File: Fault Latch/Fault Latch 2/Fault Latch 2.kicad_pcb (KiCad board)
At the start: 2 copper layers, 9 parts, among them K103 Fujitsu_FTR-LYAA005x, K104 Fujitsu_FTR-LYAA005x, K105 Fujitsu_FTR-LYAA005x, SW1 SW_Omron_B3FS, SW2 SW_Omron_B3FS, SW3 SW_Omron_B3FS, U105 SFH617A-1, U108 SFH617A-1, U111 SFH617A-1

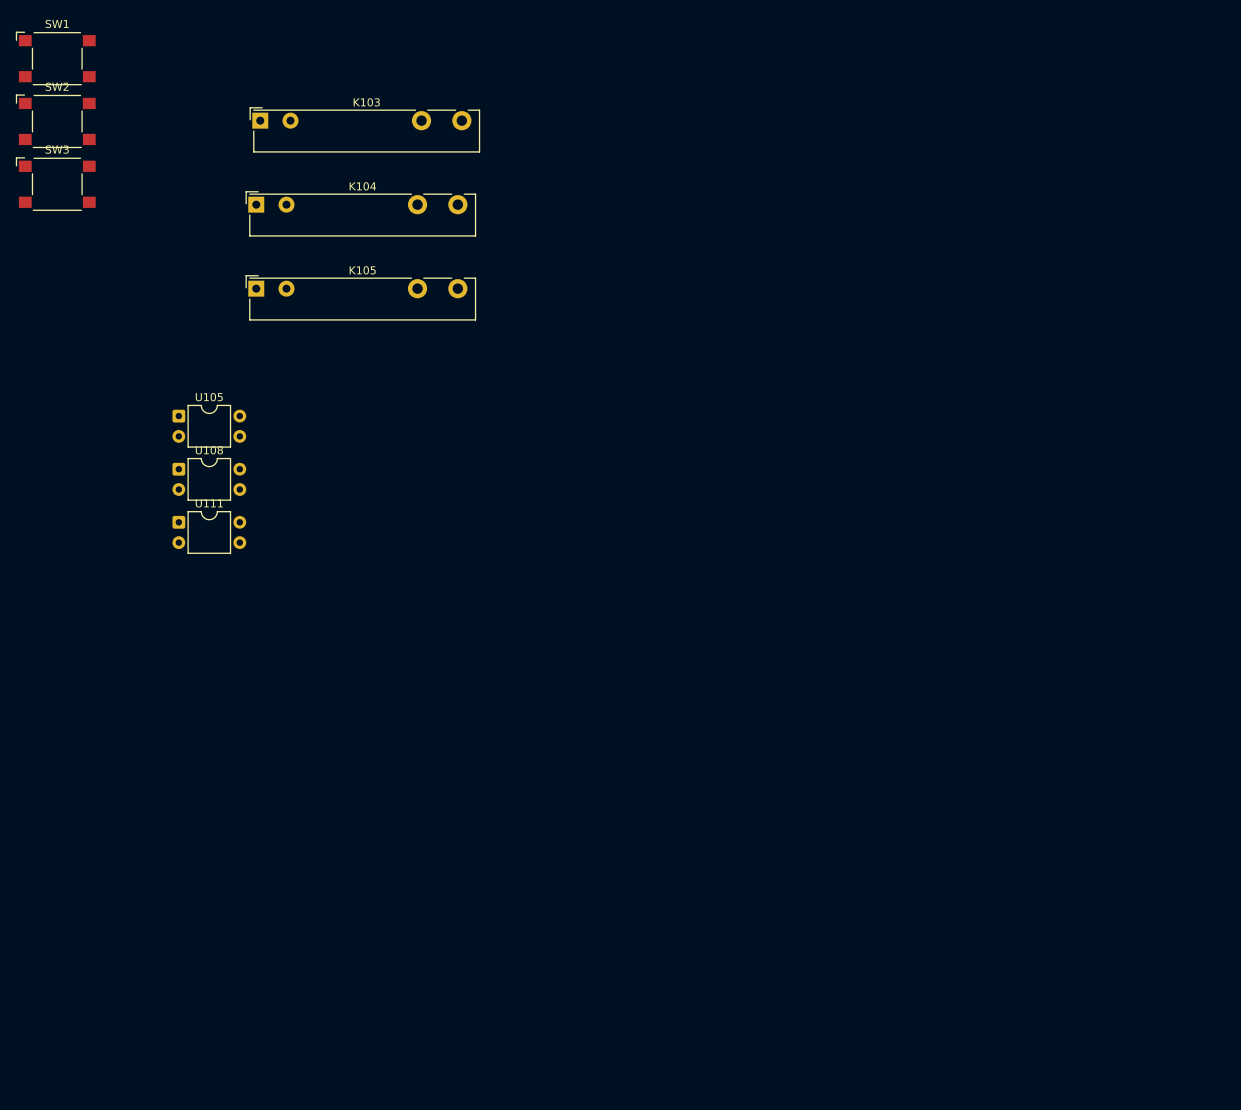
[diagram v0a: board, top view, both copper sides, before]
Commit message: Fault Latch Overhaul
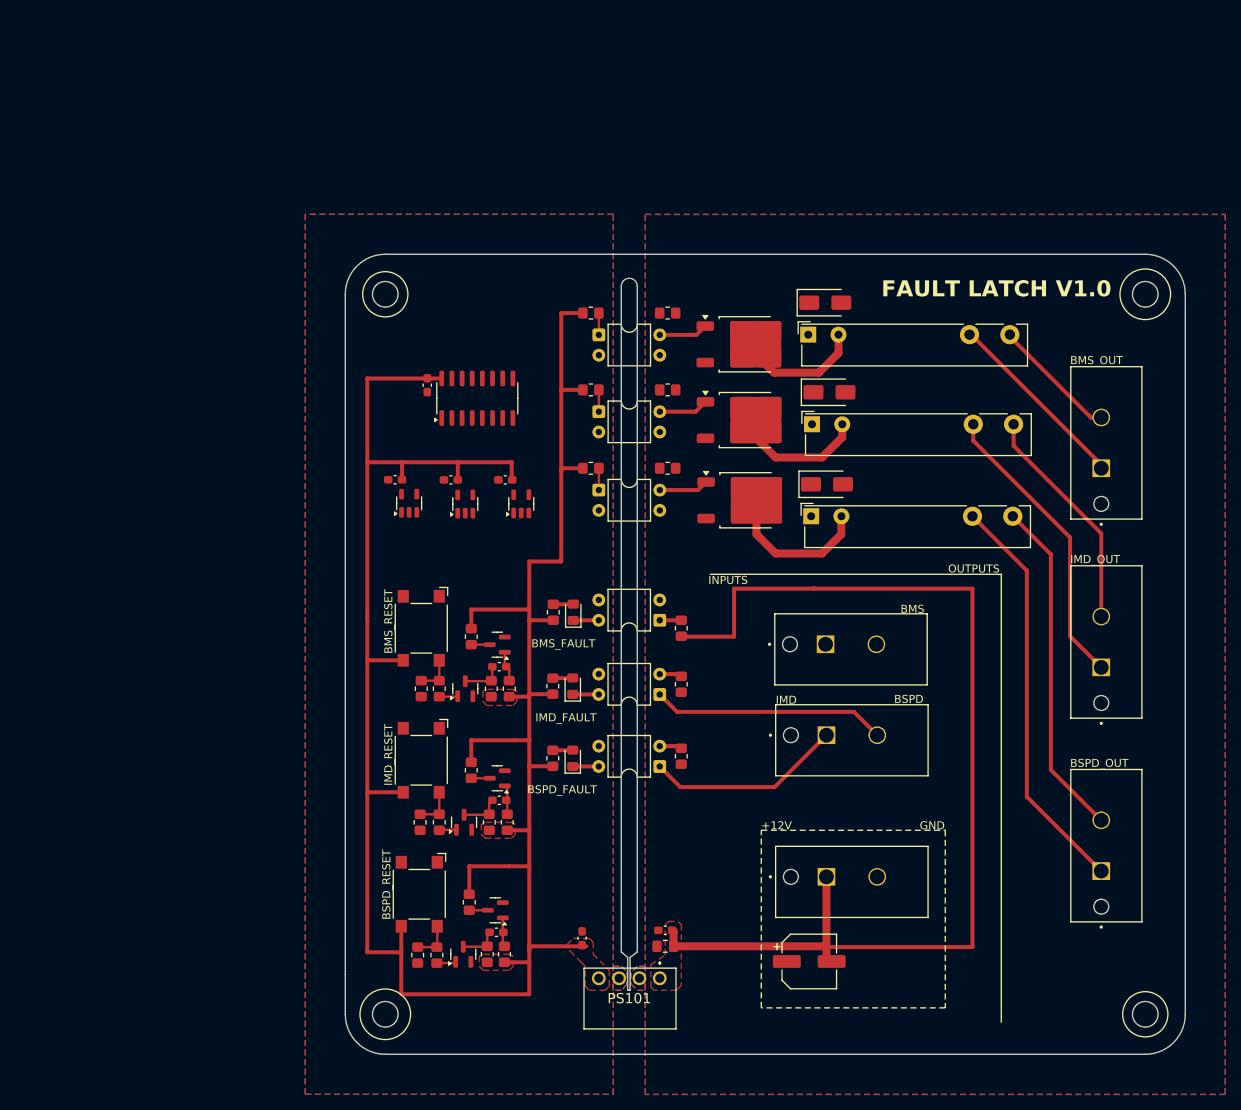
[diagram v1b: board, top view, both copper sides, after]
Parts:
- removed SW1, SW2, SW3: SW_Omron_B3FS, Button_Switch_SMD:SW_SPST_Omron_B3FS-100xP
- added C101: 10n, Capacitor_SMD:C_0603_1608Metric_Pad1.08x0.95mm_HandSolder, F.Cu at (94.2, 101.5)
- added C102: 100n, Capacitor_SMD:C_0603_1608Metric_Pad1.08x0.95mm_HandSolder, F.Cu at (88.2, 78.2)
- added C103: 100n, Capacitor_SMD:C_0603_1608Metric_Pad1.08x0.95mm_HandSolder, F.Cu at (95.0, 78.2)
- added C104: 100n, Capacitor_SMD:C_0603_1608Metric_Pad1.08x0.95mm_HandSolder, F.Cu at (81.2, 78.2)
- added C105: 10n, Capacitor_SMD:C_0603_1608Metric_Pad1.08x0.95mm_HandSolder, F.Cu at (94.2, 118.2)
- added C106: 10n, Capacitor_SMD:C_0603_1608Metric_Pad1.08x0.95mm_HandSolder, F.Cu at (93.9, 134.8)
- added C107: 47u, Capacitor_SMD:CP_Elec_6.3x5.4, F.Cu at (133.0, 138.4)
- added C108: 1u, Capacitor_SMD:C_0805_2012Metric_Pad1.18x1.45mm_HandSolder, F.Cu at (115.0, 136.5)
- added C109: 0.33u, Capacitor_SMD:C_0603_1608Metric_Pad1.08x0.95mm_HandSolder, F.Cu at (115.0, 134.5)
- added C110: 100n, Capacitor_SMD:C_0603_1608Metric_Pad1.08x0.95mm_HandSolder, F.Cu at (104.6, 135.5)
- added C111: 100n, Capacitor_SMD:C_0603_1608Metric_Pad1.08x0.95mm_HandSolder, F.Cu at (85.3, 66.4)
- added D101: RED, LED_SMD:LED_0805_2012Metric_Pad1.15x1.40mm_HandSolder, F.Cu at (103.4, 113.0)
- added D102: RED, LED_SMD:LED_0805_2012Metric_Pad1.15x1.40mm_HandSolder, F.Cu at (103.4, 104.0)
- added D103: RED, LED_SMD:LED_0805_2012Metric_Pad1.15x1.40mm_HandSolder, F.Cu at (103.5, 94.8)
- added D104: D_Schottky, Diode_SMD:D_SMA, F.Cu at (135.0, 56.0)
- added D105: D_Schottky, Diode_SMD:D_SMA, F.Cu at (135.5, 67.2)
- added D106: D_Schottky, Diode_SMD:D_SMA, F.Cu at (135.2, 78.8)
- added H101: MountingHole, MountingHole:MountingHole_3.2mm_M3, F.Cu at (80.0, 145.0)
- added H102: MountingHole, MountingHole:MountingHole_3.2mm_M3, F.Cu at (175.0, 145.0)
- added H103: MountingHole, MountingHole:MountingHole_3.2mm_M3, F.Cu at (175.0, 55.0)
- added H104: MountingHole, MountingHole:MountingHole_3.2mm_M3, F.Cu at (80.0, 55.0)
- added PS101: RI-1205S, DC-DC:RI0505S, F.Cu at (114.3, 140.5)
- added Q104: Q_NPN_BEC, Package_TO_SOT_SMD:SOT-23, F.Cu at (90.0, 104.3)
- added Q106: Q_NPN_BEC, Package_TO_SOT_SMD:SOT-23, F.Cu at (94.0, 98.8)
- added Q107: Q_NPN_BEC, Package_TO_SOT_SMD:SOT-23, F.Cu at (89.8, 121.0)
- added Q108: Q_NPN_BEC, Package_TO_SOT_SMD:SOT-23, F.Cu at (94.0, 115.5)
- added Q109: Q_NMOS_GDS, Package_TO_SOT_SMD:TO-252-2, F.Cu at (125.0, 61.2)
- added Q110: Q_NMOS_GDS, Package_TO_SOT_SMD:TO-252-2, F.Cu at (125.1, 70.7)
- added Q111: Q_NMOS_GDS, Package_TO_SOT_SMD:TO-252-2, F.Cu at (125.1, 80.8)
- added Q112: Q_NPN_BEC, Package_TO_SOT_SMD:SOT-23, F.Cu at (89.8, 137.5)
- added Q113: Q_NPN_BEC, Package_TO_SOT_SMD:SOT-23, F.Cu at (93.8, 132.0)
- added R101: 100k, Resistor_SMD:R_0805_2012Metric_Pad1.20x1.40mm_HandSolder, F.Cu at (84.5, 104.3)
- added R102: 10k, Resistor_SMD:R_0805_2012Metric_Pad1.20x1.40mm_HandSolder, F.Cu at (86.8, 104.3)
- added R104: 270R, Resistor_SMD:R_0805_2012Metric_Pad1.20x1.40mm_HandSolder, F.Cu at (100.9, 113.0)
- added R105: 270R, Resistor_SMD:R_0805_2012Metric_Pad1.20x1.40mm_HandSolder, F.Cu at (100.9, 104.0)
- added R106: 1k, Resistor_SMD:R_0805_2012Metric_Pad1.20x1.40mm_HandSolder, F.Cu at (93.2, 104.3)
- added R107: 270R, Resistor_SMD:R_0805_2012Metric_Pad1.20x1.40mm_HandSolder, F.Cu at (101.0, 94.8)
- added R108: 100k, Resistor_SMD:R_0805_2012Metric_Pad1.20x1.40mm_HandSolder, F.Cu at (95.5, 104.3)
- added R109: 1k, Resistor_SMD:R_0805_2012Metric_Pad1.20x1.40mm_HandSolder, F.Cu at (90.8, 97.8)
- added R112: 100k, Resistor_SMD:R_0805_2012Metric_Pad1.20x1.40mm_HandSolder, F.Cu at (84.3, 121.0)
- added R113: 10k, Resistor_SMD:R_0805_2012Metric_Pad1.20x1.40mm_HandSolder, F.Cu at (86.8, 121.0)
- added R114: 1k, Resistor_SMD:R_0805_2012Metric_Pad1.20x1.40mm_HandSolder, F.Cu at (93.0, 121.0)
- added R115: 100k, Resistor_SMD:R_0805_2012Metric_Pad1.20x1.40mm_HandSolder, F.Cu at (95.2, 121.0)
- added R116: 270R, Resistor_SMD:R_0805_2012Metric_Pad1.20x1.40mm_HandSolder, F.Cu at (105.7, 57.4)
- added R117: 270R, Resistor_SMD:R_0805_2012Metric_Pad1.20x1.40mm_HandSolder, F.Cu at (105.7, 67.0)
- added R118: 270R, Resistor_SMD:R_0805_2012Metric_Pad1.20x1.40mm_HandSolder, F.Cu at (105.7, 76.8)
- added R120: 1k, Resistor_SMD:R_0805_2012Metric_Pad1.20x1.40mm_HandSolder, F.Cu at (90.8, 114.5)
- added R121: 10k, Resistor_SMD:R_0805_2012Metric_Pad1.20x1.40mm_HandSolder, F.Cu at (115.3, 57.4)
- added R122: 10k, Resistor_SMD:R_0805_2012Metric_Pad1.20x1.40mm_HandSolder, F.Cu at (115.3, 67.0)
- added R123: 10k, Resistor_SMD:R_0805_2012Metric_Pad1.20x1.40mm_HandSolder, F.Cu at (115.3, 76.8)
- added R124: 100k, Resistor_SMD:R_0805_2012Metric_Pad1.20x1.40mm_HandSolder, F.Cu at (84.0, 137.6)
- added R125: 10k, Resistor_SMD:R_0805_2012Metric_Pad1.20x1.40mm_HandSolder, F.Cu at (86.5, 137.6)
- added R126: 1k, Resistor_SMD:R_0805_2012Metric_Pad1.20x1.40mm_HandSolder, F.Cu at (92.8, 137.5)
- added R127: 100k, Resistor_SMD:R_0805_2012Metric_Pad1.20x1.40mm_HandSolder, F.Cu at (94.9, 137.5)
- added R128: 1k, Resistor_SMD:R_0805_2012Metric_Pad1.20x1.40mm_HandSolder, F.Cu at (90.5, 131.0)
- added R129: 10k, Resistor_SMD:R_0805_2012Metric_Pad1.20x1.40mm_HandSolder, F.Cu at (117.0, 96.8)
- added R131: 2.2k, Resistor_SMD:R_0805_2012Metric_Pad1.20x1.40mm_HandSolder, F.Cu at (117.0, 112.8)
- added R135: 10k, Resistor_SMD:R_0805_2012Metric_Pad1.20x1.40mm_HandSolder, F.Cu at (117.0, 103.8)
- added SW101: SW_Omron_B3FS, Button_Switch_SMD:SW_SPST_Omron_B3FS-100xP, F.Cu at (84.5, 96.8)
- added SW102: SW_Omron_B3FS, Button_Switch_SMD:SW_SPST_Omron_B3FS-100xP, F.Cu at (84.5, 113.2)
- added SW103: SW_Omron_B3FS, Button_Switch_SMD:SW_SPST_Omron_B3FS-100xP, F.Cu at (84.2, 130.0)
- added U101: 641964-1, 641964-1:TE_641964-1, F.Cu at (135.0, 98.8)
- added U102: 74AHC1G00, Package_TO_SOT_SMD:SOT-23-5, F.Cu at (83.0, 81.1)
- added U103: 74AHC1G00, Package_TO_SOT_SMD:SOT-23-5, F.Cu at (90.0, 81.2)
- added U104: 74AHC1G00, Package_TO_SOT_SMD:SOT-23-5, F.Cu at (97.0, 81.2)
- added U105: 641964-1, 641964-1:TE_641964-1, F.Cu at (135.2, 110.1)
- added U106: 74LS279, Package_SO:SOIC-16_3.9x9.9mm_P1.27mm, F.Cu at (91.5, 68.0)
- added U110: 641964-1, 641964-1:TE_641964-1, F.Cu at (169.5, 76.8)
- added U111: 641964-1, 641964-1:TE_641964-1, F.Cu at (169.5, 101.6)
- added U112: 641964-1, 641964-1:TE_641964-1, F.Cu at (169.5, 127.1)
- added U113: 641964-1, 641964-1:TE_641964-1, F.Cu at (135.1, 127.8)
- added U114: SFH617A-1, Package_DIP:DIP-4_W7.62mm, F.Cu at (114.3, 95.8)
- added U115: SFH617A-1, Package_DIP:DIP-4_W7.62mm, F.Cu at (114.3, 114.0)
- added U116: SFH617A-1, Package_DIP:DIP-4_W7.62mm, F.Cu at (114.3, 105.0)
- moved K103 75.0 mm to (133.2, 82.8)
- moved K102 74.7 mm to (133.3, 71.2)
- moved K101 73.5 mm to (132.9, 60.0)
- moved U107 53.5 mm to (106.7, 60.1)
- moved U108 53.0 mm to (106.7, 69.7)
- moved U109 52.7 mm to (106.7, 79.5)
- renumbered K103 to K101, K104 to K102, K105 to K103, U105 to U107, U111 to U109
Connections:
- net GND renamed GNDPWR
- K103 pad 13: unconnected-(K105-Pad13) -> Net-(K103-Pad13)
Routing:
- net +5V: track 0.00 -> 296.7 mm
- net +12V: track 0.00 -> 138.4 mm
- net Net-(K103-Pad13): track 0.00 -> 51.0 mm
- net Net-(K103-Pad14): track 0.00 -> 42.6 mm
- net Net-(K102-Pad13): track 0.00 -> 37.0 mm
- net /BSPD_HV: track 0.00 -> 29.3 mm
- net Net-(K102-Pad14): track 0.00 -> 28.6 mm
- net /IMD_HV: track 0.00 -> 24.6 mm
- net Net-(K101-Pad13): track 0.00 -> 23.6 mm
- net Net-(D106-A): track 0.00 -> 19.1 mm
- net Net-(D105-A): track 0.00 -> 16.7 mm
- net Net-(D104-A): track 0.00 -> 15.9 mm
- net Net-(K101-Pad14): track 0.00 -> 15.8 mm
- net Net-(Q110-G): track 0.00 -> 6.22 mm
- net Net-(Q111-G): track 0.00 -> 6.20 mm
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- added copper zone on F.Cu, net +12V
- added copper zone on F.Cu, net +5V
- added copper zone on B.Cu, net GND
- added copper zone on F.Cu, net GND
- added copper zone on B.Cu, net GNDPWR
- added copper zone on F.Cu, net GNDPWR
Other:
- board outline added: 105 x 100 mm
- board text added: "+12V"
- board text added: "BMS"
- board text added: "BMS_FAULT"
- board text added: "BMS_OUT"
- board text added: "BMS_RESET"
- board text added: "BSPD"
- board text added: "BSPD_FAULT"
- board text added: "BSPD_OUT"
- board text added: "BSPD_RESET"
- board text added: "FAULT LATCH V1.0"
- board text added: "GND"
- board text added: "IMD"
- board text added: "IMD_FAULT"
- board text added: "IMD_OUT"
- board text added: "IMD_RESET"
- board text added: "INPUTS"
- board text added: "OUTPUTS"
